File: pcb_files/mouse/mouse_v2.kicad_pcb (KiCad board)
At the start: 2 copper layers, 94.8 x 94.9 mm, 49 parts, among them J4 I2C_Conn, M1 Motor_DC, M2 Motor_DC, M3 CASTER_BALL, Q0 Q_Photo_NPN, Q1 Q_Photo_NPN, Q2 Q_Photo_NPN, Q3 Q_Photo_NPN, T0 Q_NMOS_DGS, T1 Q_NMOS_DGS, T2 Q_NMOS_DGS, T3 Q_NMOS_DGS, U1 Teensy4.0, U2 SN754410NE, U3 LM1085-5.0, U4 Encoder_3081, U5 Encoder_3081

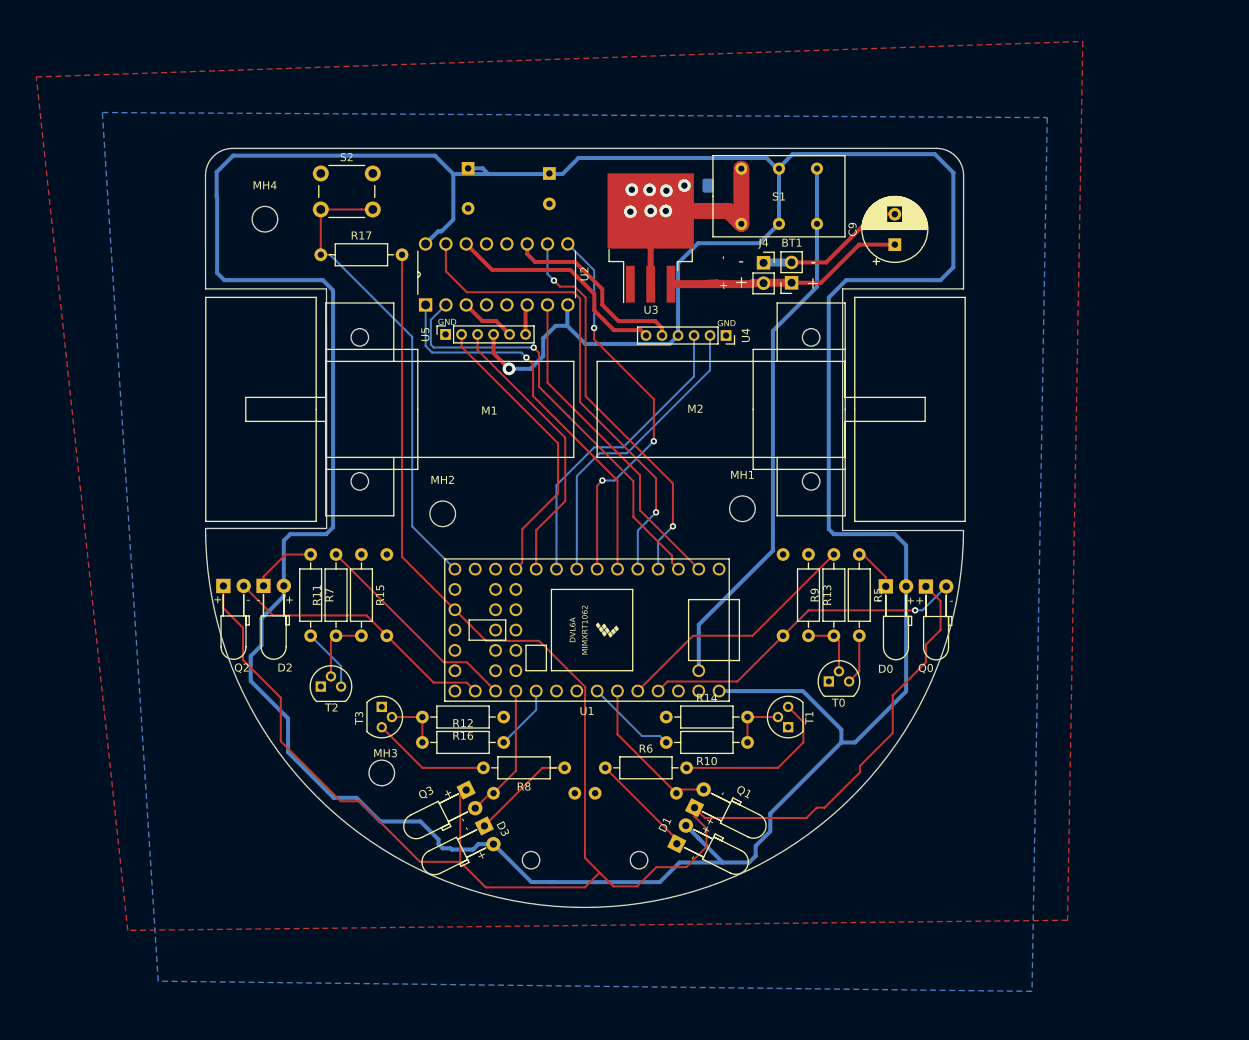
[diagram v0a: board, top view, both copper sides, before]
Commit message: Slimmed Model
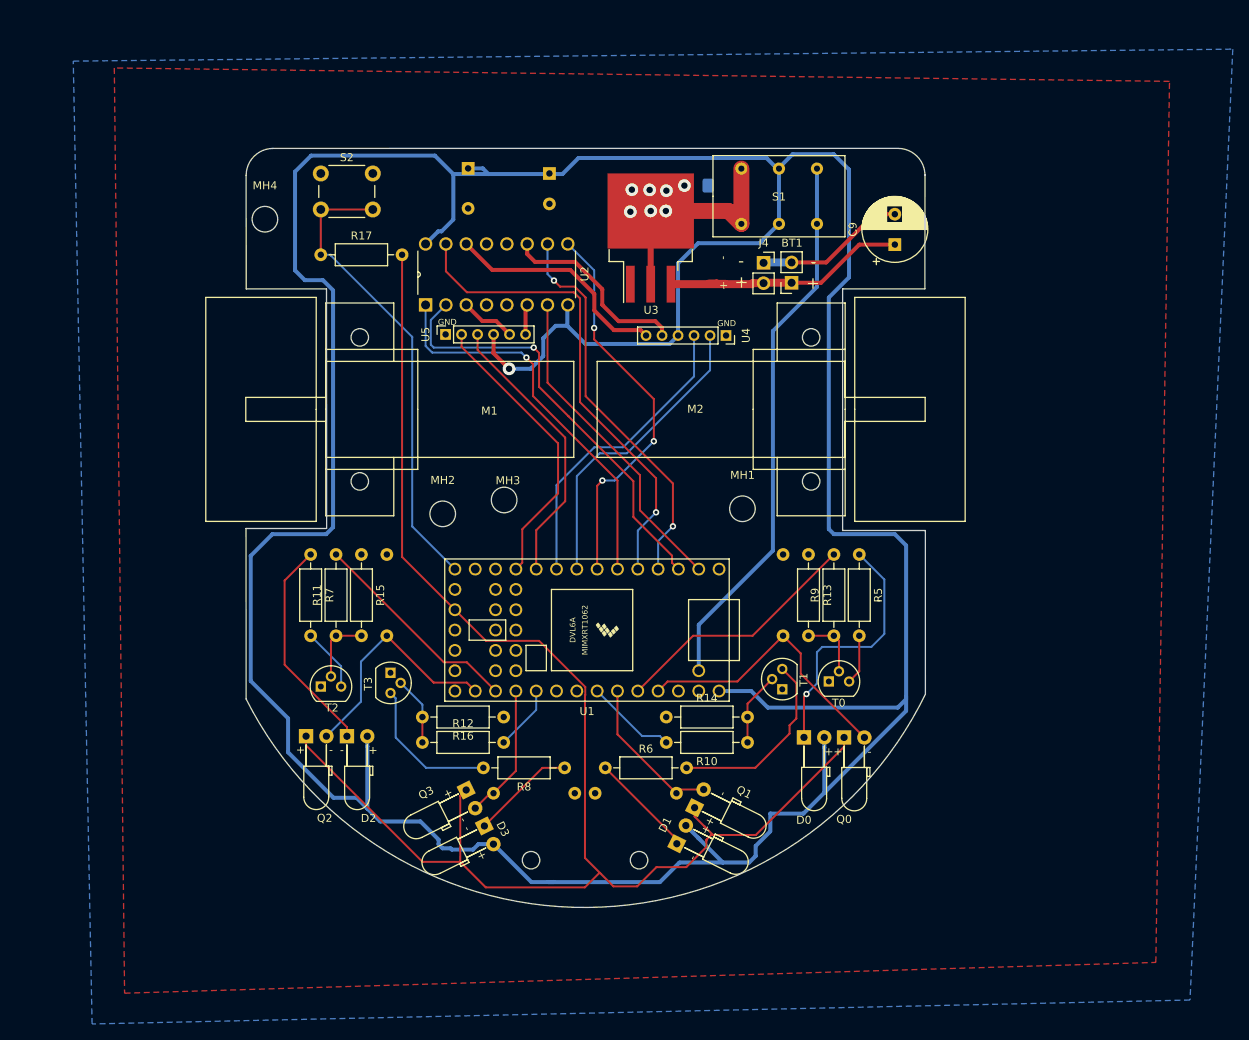
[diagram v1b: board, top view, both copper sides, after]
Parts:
- moved MH3 37.4 mm to (149.9, 98.6)
- moved D2 21.5 mm to (130.3, 128.1)
- moved D0 21.5 mm to (187.4, 128.3)
- moved Q0 21.5 mm to (192.4, 128.3)
- moved Q2 21.4 mm to (125.2, 128.1)
- moved T1 4.80 mm to (184.7, 122.3)
- moved T3 4.40 mm to (135.7, 120.2)
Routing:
- net /3.3v: track 244.6 -> 192.1 mm
- net Net-(D0-Pad1): track 5.87 -> 32.4 mm, vias 0 -> 1
- net /5v: track 480.2 -> 460.1 mm
- net Net-(D2-Pad1): track 8.19 -> 27.3 mm
- net /Reciever_0: track 41.4 -> 35.4 mm, vias 1 -> 0
- net /Reciever_2: track 34.4 -> 29.6 mm
- net Net-(R8-Pad2): track 14.8 -> 18.4 mm
- net Net-(R6-Pad2): track 21.2 -> 23.8 mm
- net Net-(R10-Pad1): track 6.98 -> 9.19 mm
- net Net-(R12-Pad1): track 6.98 -> 8.57 mm
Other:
- board size 94.8 x 94.9 mm -> 84.9 x 94.9 mm

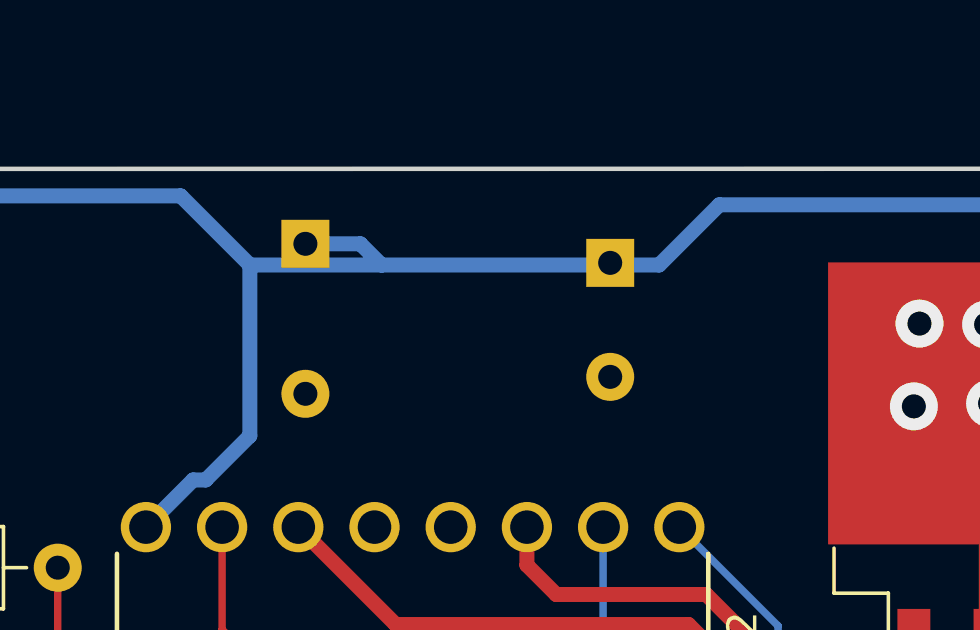
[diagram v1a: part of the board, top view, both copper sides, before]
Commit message: deleted files in fish-mouse folder
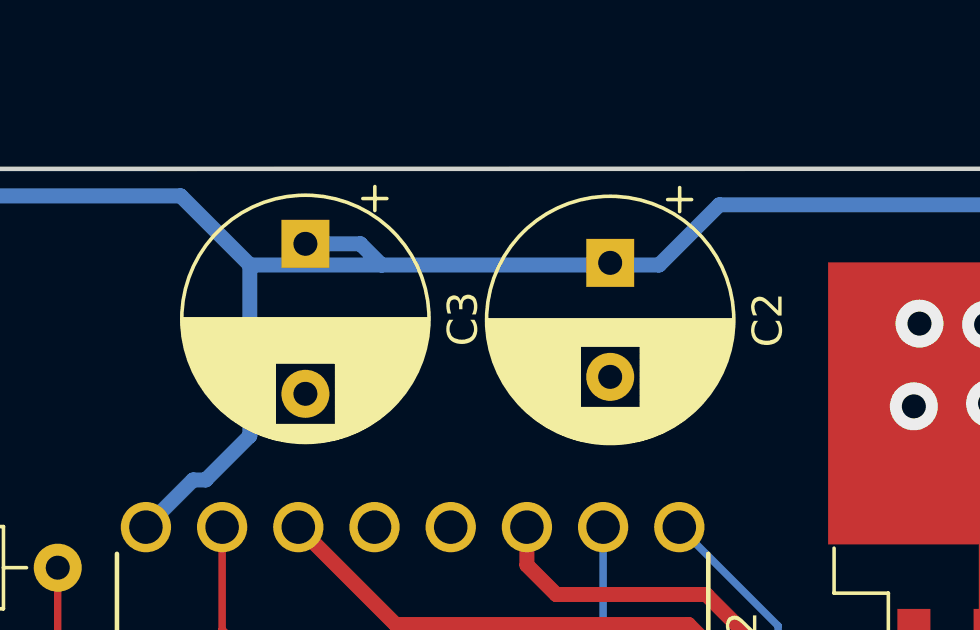
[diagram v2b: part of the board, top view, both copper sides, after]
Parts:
- C2, C3: moved to F.Cu

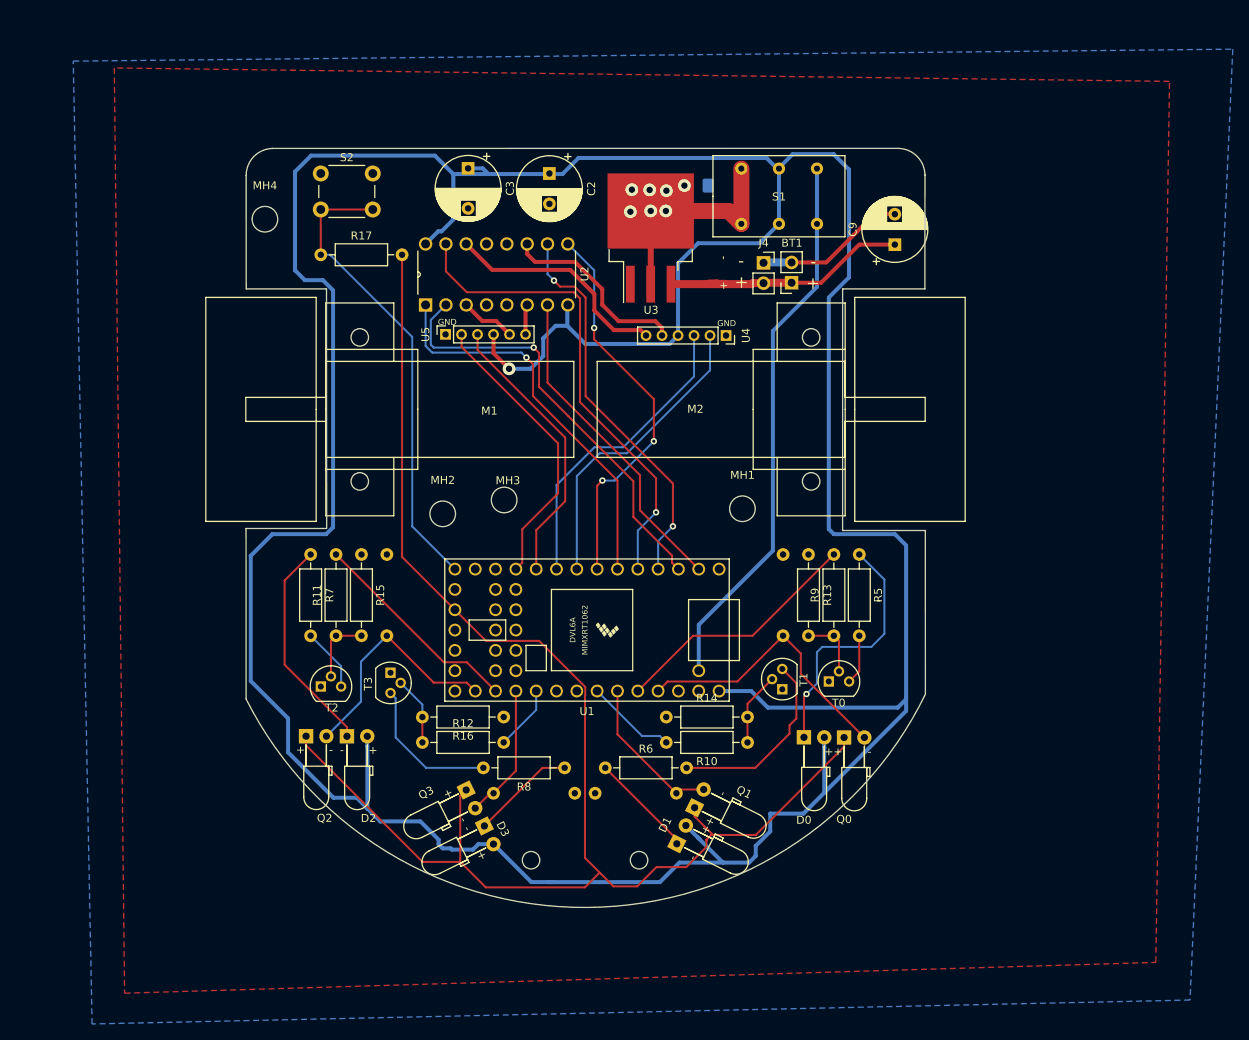
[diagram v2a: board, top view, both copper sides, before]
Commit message: SMD Caps, Space for Skates, Smaller Switch
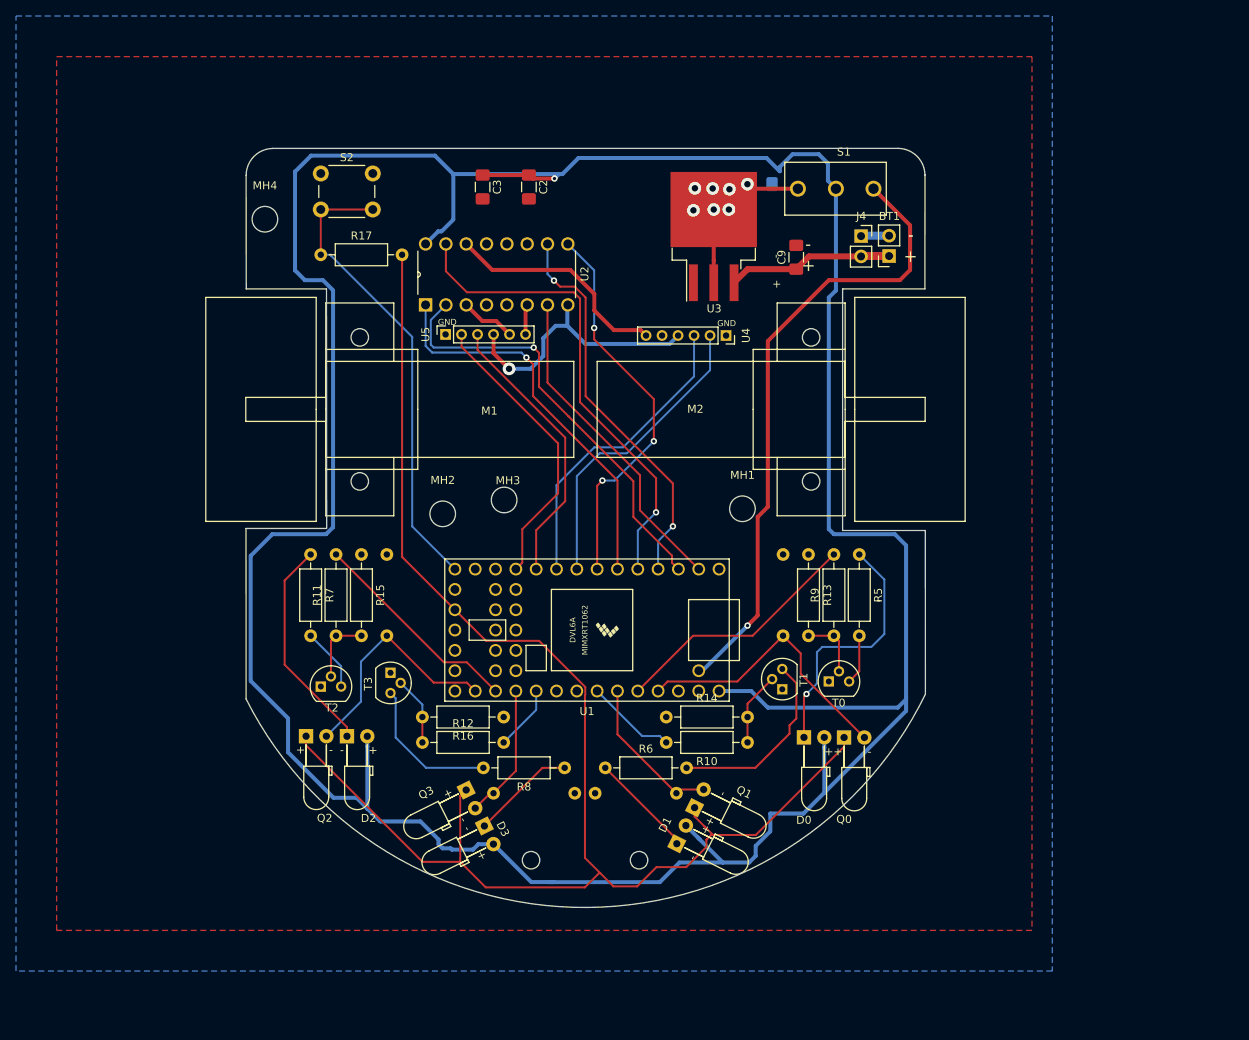
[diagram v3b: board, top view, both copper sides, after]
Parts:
- C2, C9: footprint Capacitor_THT:CP_Radial_D8.0mm_P3.80mm -> Capacitor_SMD:C_1206_3216Metric_Pad1.42x1.75mm_HandSolder
- C3: footprint Capacitor_THT:CP_Radial_D8.0mm_P5.00mm -> Capacitor_SMD:C_1206_3216Metric_Pad1.42x1.75mm_HandSolder
- S1: footprint misc:PW_SLIDE_SW -> misc:SWITCH_SLIDE_500SSP1S2M2QEA
- moved BT1 12.6 mm to (198.0, 68.1)
- moved J4 12.6 mm to (194.5, 65.6)
- moved C9 12.4 mm to (186.4, 68.3)
- moved C10 7.98 mm to (181.9, 59.1)
- moved U3 7.88 mm to (176.1, 65.7)
- moved C2 3.07 mm to (153.0, 59.5)
- moved C3 2.95 mm to (147.2, 59.5)
- moved S1 2.59 mm to (186.7, 59.7), turned to 0 degrees
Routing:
- net /5v: track 460.1 -> 434.6 mm, vias 1 -> 2
- net /OUT3: track 24.0 -> 0.00 mm
- net /GND: track 18.9 -> 3.53 mm
- net /vBatt: track 32.2 -> 21.3 mm
- net /VUSB: track 68.9 -> 78.6 mm, vias 0 -> 1
- net Net-(C10-Pad1): track 31.6 -> 22.9 mm
